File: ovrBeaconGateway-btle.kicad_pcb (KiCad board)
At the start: 2 copper layers, 31.1 x 44.7 mm, 27 parts, among them J1 CONN_RJ45_RA, J2 CONN_1.27MM_5X2, Q1 FET_N_1.2A_20V, Q2 FET_N_1.2A_20V, U1 SILICONLABS_SI7050, U2 TOREX_XC6210, U3 LITEON_LTR-329ALS, U4 INTERSIL_ISL32602EFBZ, U5 BLUEGIGA_BLE121

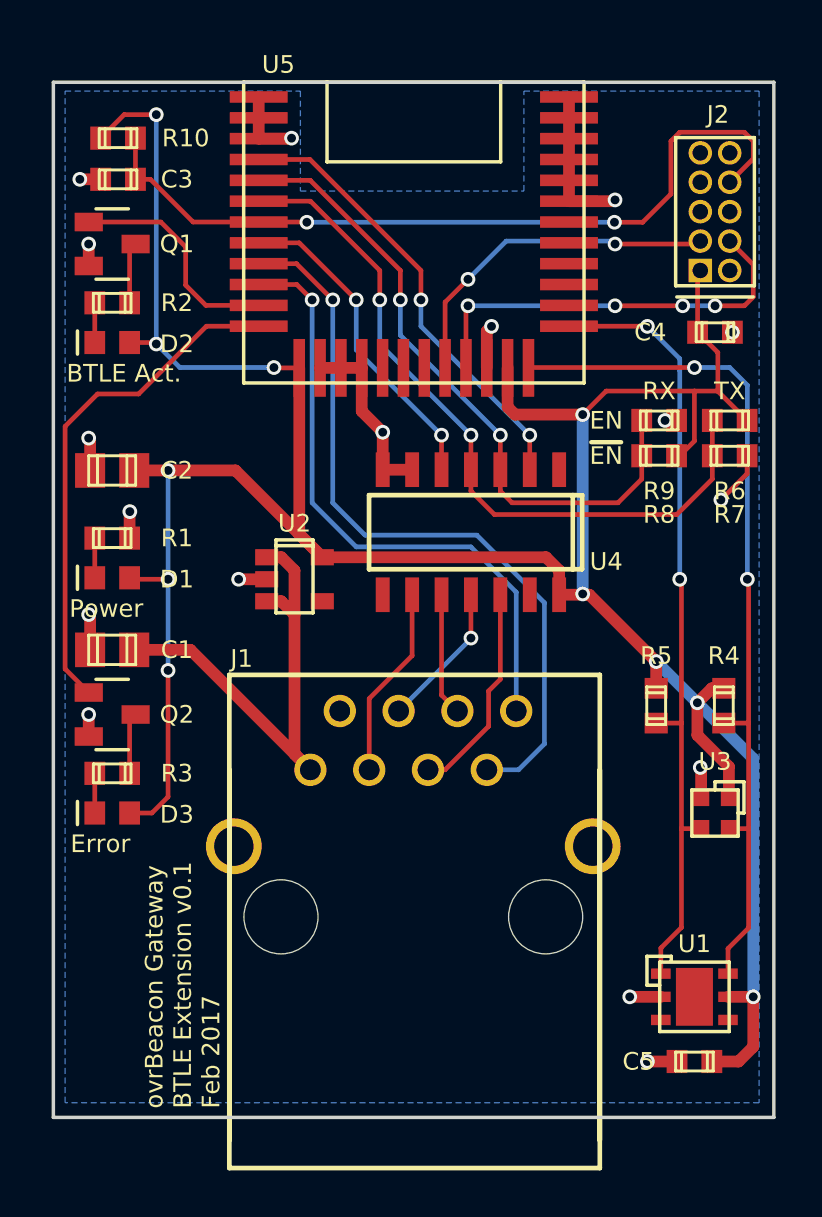
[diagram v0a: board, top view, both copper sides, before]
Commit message: Out for DFM
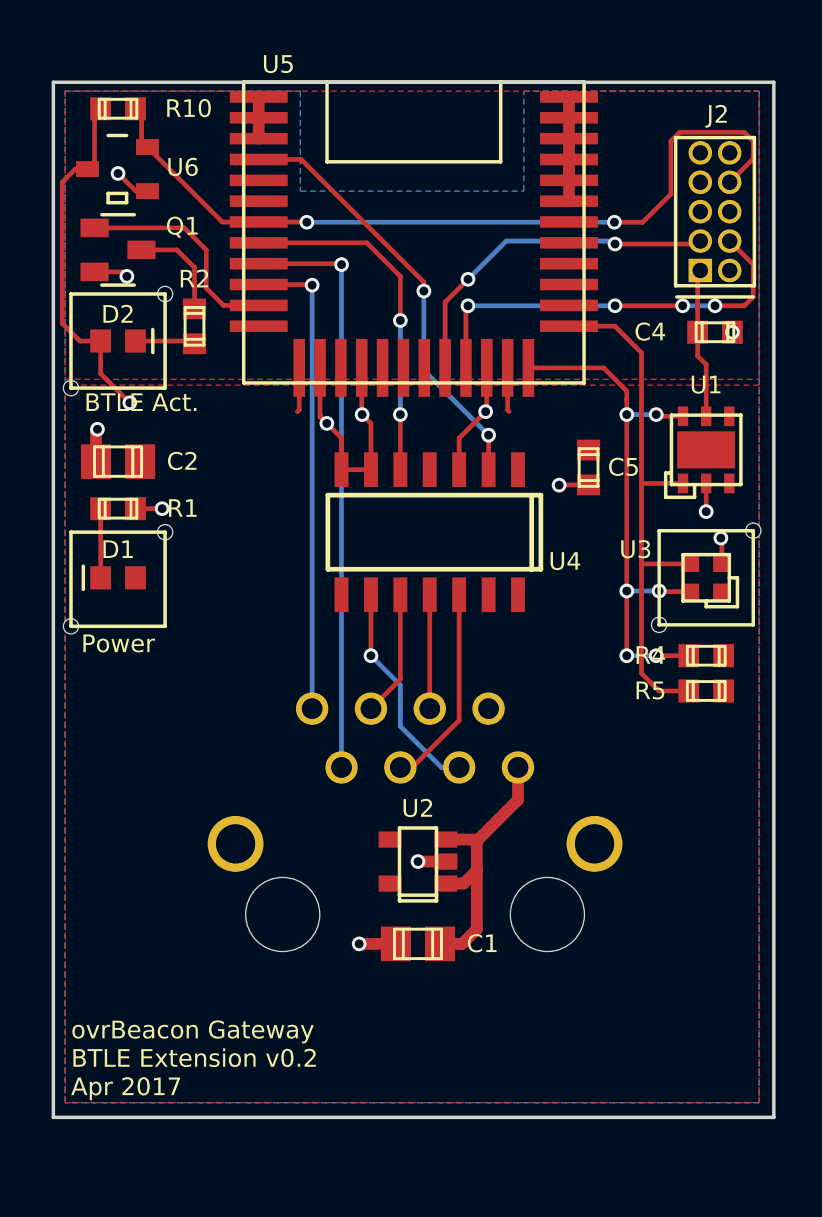
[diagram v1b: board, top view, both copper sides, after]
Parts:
- removed C3: C_10000pF_25v_0603, ovrEngineered:C_0603
- removed D3: LED_RED_0603, ovrEngineered:D_0603
- removed Q2: FET_N_1.2A_20V, ovrEngineered:FET_N_1.2A_20V
- removed R3: R_402_1%_0603, ovrEngineered:R_0603
- removed R6, R7, R8, R9: R_10K_1%_0603, ovrEngineered:R_0603
- added REF**: LIGHTPIPE_VLP-XXX, ovrEngineered:LIGHTPIPE_VLP-XXX, F.Cu at (132.3, 64.4)
- added REF**: LIGHTPIPE_VLP-XXX, ovrEngineered:LIGHTPIPE_VLP-XXX, F.Cu at (132.3, 74.7)
- added REF**: LIGHTPIPE_VLP-XXX, ovrEngineered:LIGHTPIPE_VLP-XXX, F.Cu at (157.7, 74.6)
- added U6: MIC803-29D4VM3, ovrEngineered:SOT-23-3, F.Cu at (133.6, 57.9)
- J1: moved to B.Cu
- moved C5 26.1 mm to (152.7, 69.8), turned to 90 degrees
- moved U1 23.6 mm to (157.7, 69.1), turned to 90 degrees
- moved C1 18.3 mm to (145.3, 90.4)
- moved U2 13.3 mm to (145.3, 86.9), turned to 180 degrees
- moved U3 10.2 mm to (157.7, 74.6), turned to 180 degrees
- moved J1 8.97 mm to (149.6, 82.8), turned to 180 degrees
- moved R2 3.70 mm to (135.6, 63.8), turned to 90 degrees
- moved R4 2.29 mm to (157.7, 78.0), turned to 0 degrees
- moved R5 2.25 mm to (157.7, 79.5), turned to 0 degrees
- moved U4 1.78 mm to (145.8, 72.6)
- moved R1 1.30 mm to (132.3, 71.6)
- moved R10 1.27 mm to (132.3, 54.4)
- moved C2 0.46 mm to (132.3, 69.6)
- moved Q1 0.36 mm to (132.3, 60.5)
- moved D2 0.26 mm to (132.3, 64.4), turned to 180 degrees
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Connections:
- U4 pad 3: /~422_RE -> GND
- U4 pad 4: /422_DE -> +3V3
- U5 pad 12: /LED_ERROR -> (no net)
- U5 pad 15: GND -> (no net)
- U5 pad 5: /~422_RE -> (no net)
- U5 pad 6: /422_DE -> (no net)
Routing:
- net +3V3: track 131.8 -> 25.9 mm, vias 11 -> 1
- net /422_DE: track 31.6 -> 0.00 mm, vias 2 -> 0
- net /~422_RE: track 28.3 -> 0.00 mm, vias 2 -> 0
- net /LED_ERROR: track 22.1 -> 0.00 mm
- net /SCL: track 37.5 -> 24.0 mm, vias 2 -> 6
- net /SDA: track 34.3 -> 23.7 mm, vias 2 -> 0
- net +5V: track 21.5 -> 12.5 mm
- net /BLE121-CTS: track 32.6 -> 25.3 mm
- net /BLE121-RTS: track 26.9 -> 20.6 mm
- net Net-(Q2-Pad3): track 2.65 -> 0.00 mm
- net Net-(Q1-Pad3): track 2.65 -> 4.39 mm
- net Net-(D3-Pad2): track 1.71 -> 0.00 mm
- net Net-(J1-Pad4): track 6.32 -> 4.92 mm, vias 1 -> 0
- net Net-(D1-Pad2): track 1.71 -> 2.98 mm
- net Net-(J1-Pad3): track 8.33 -> 9.48 mm, vias 0 -> 1
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- added copper zone on F.Cu, net +3V3
- added copper zone on F.Cu, net GND
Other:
- board text added: "ovrBeacon Gateway BTLE Extension v0.2 Apr 2017"
- board text removed: "EN"
- board text removed: "Error"
- board text removed: "RX"
- board text removed: "TX"
- board text removed: "ovrBeacon Gateway BTLE Extension v0.1 Feb 2017"
- board text removed: "~EN"
